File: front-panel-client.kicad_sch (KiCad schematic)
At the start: 9 parts, among them IC16 PMV20ENR, IC18 PMV20ENR, J4 855-M50-3500542

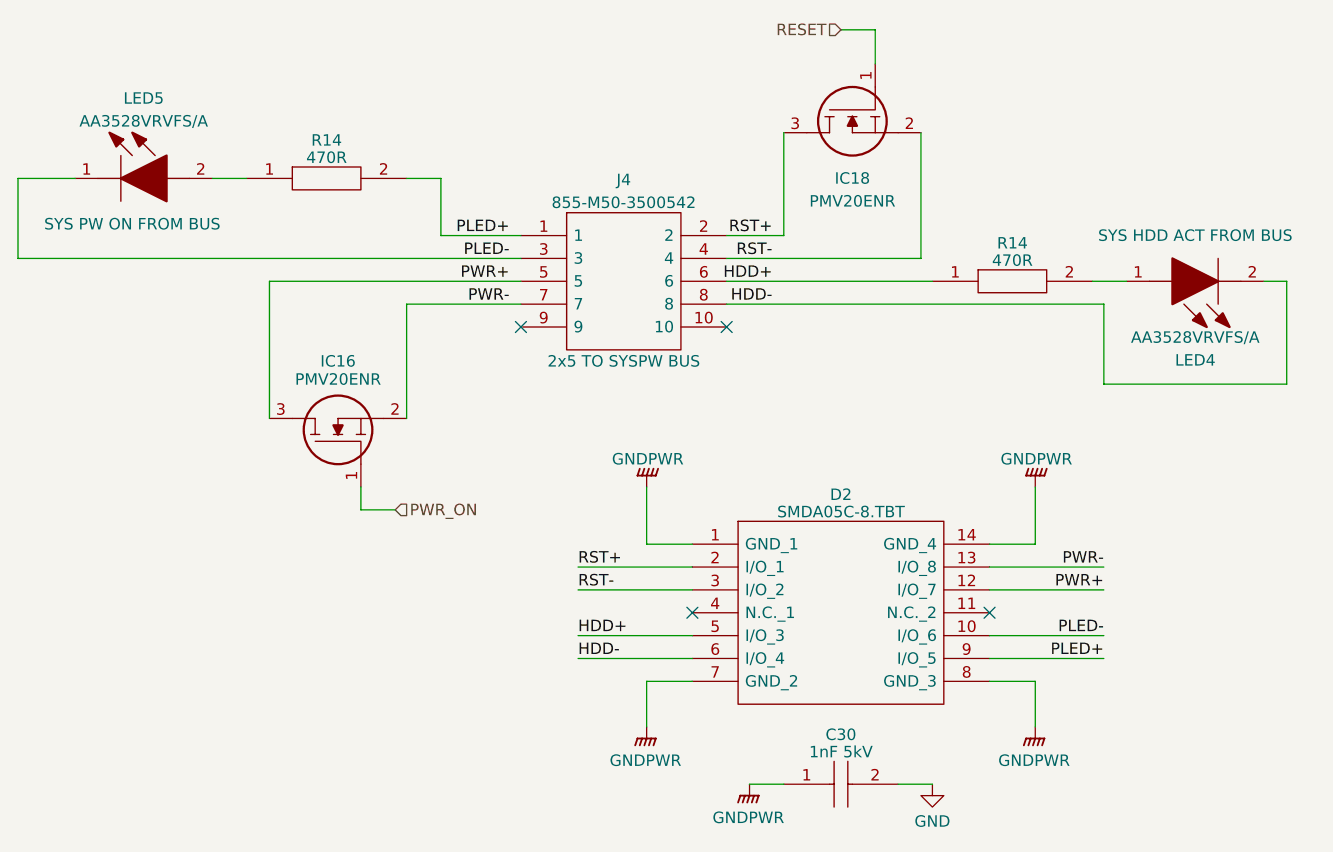
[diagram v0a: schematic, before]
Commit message: first round of revisions
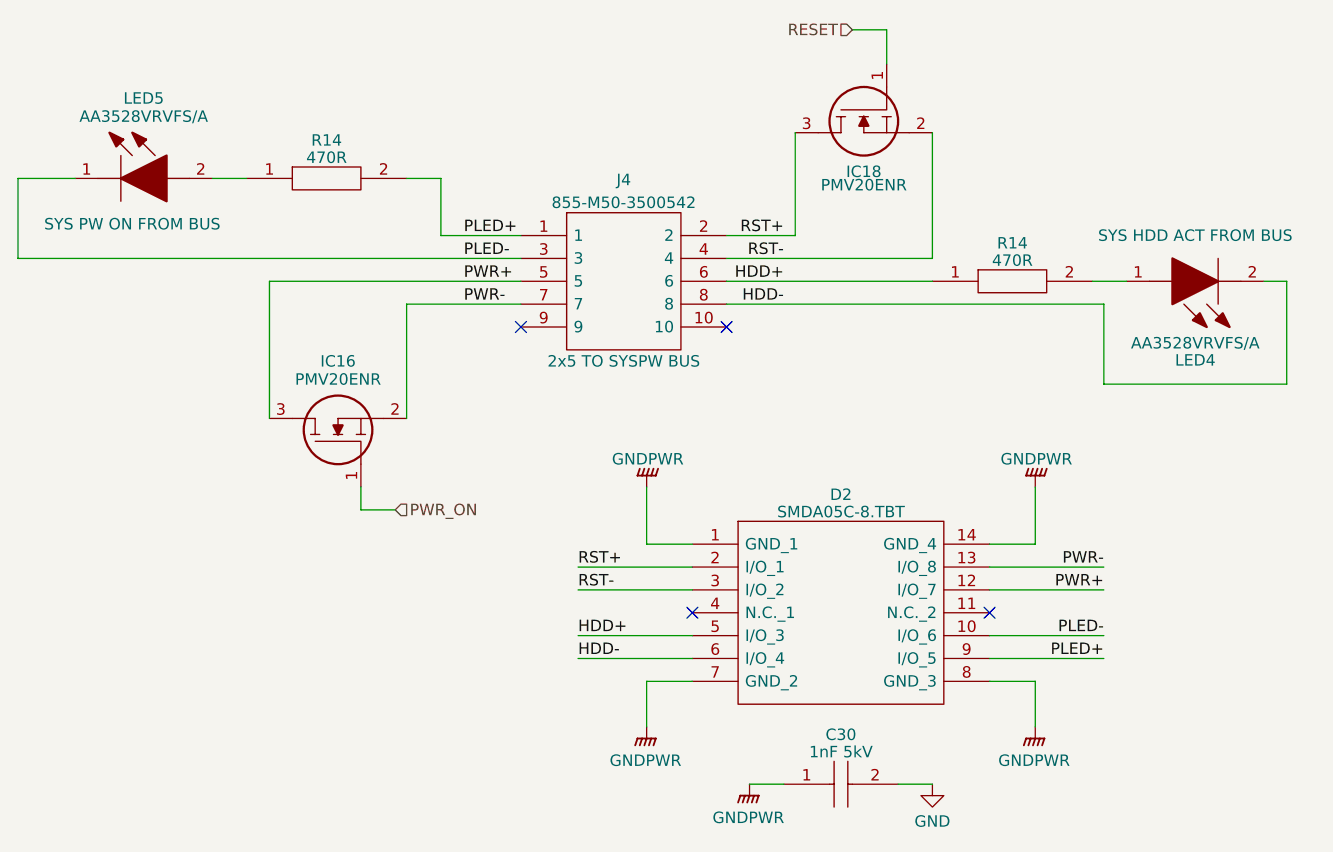
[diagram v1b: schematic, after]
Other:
- moved on the sheet: IC18
